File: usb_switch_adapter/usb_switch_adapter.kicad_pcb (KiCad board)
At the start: 2 copper layers, 19.4 x 33.3 mm, 12 parts, among them J1 USB-C Plug, J2 USB2.0-C_SMT, M2 Hole_M2_2.0, SW1 SW_Push, U1 CH217K, U2 CH32V003J4M6

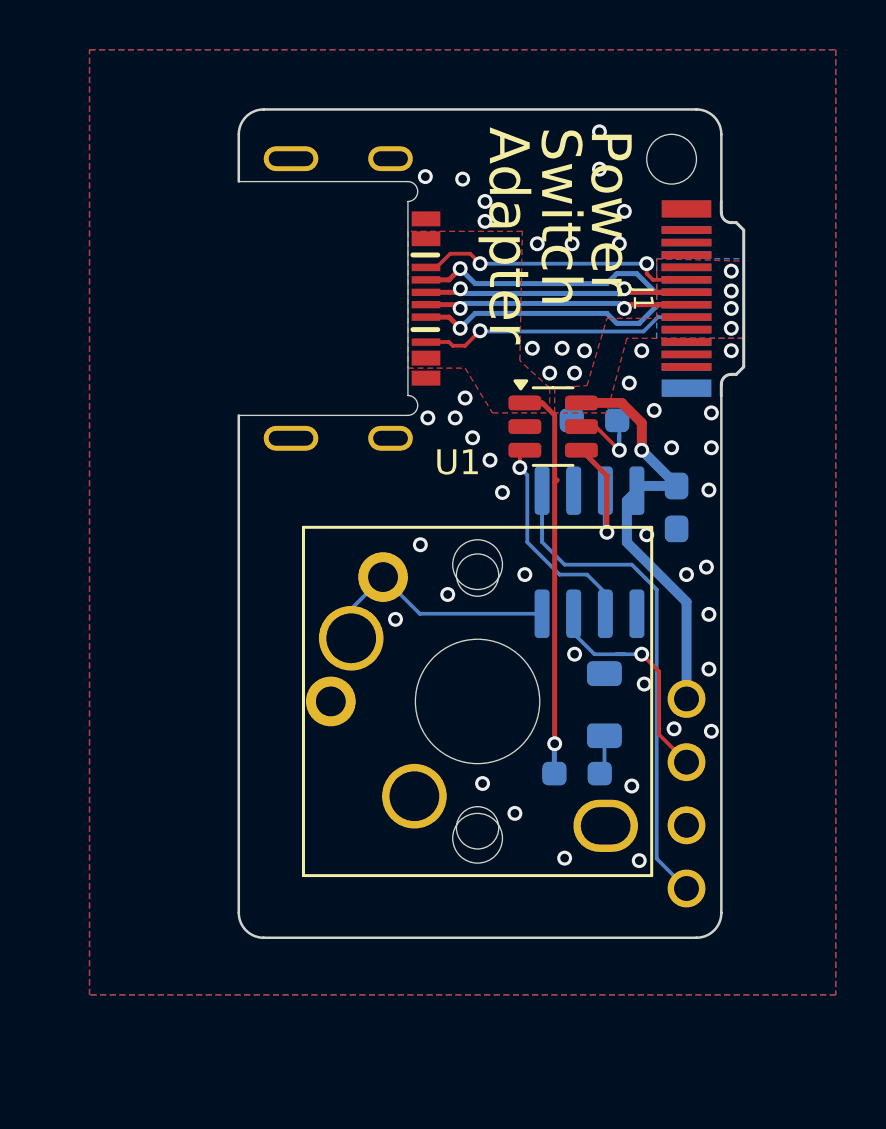
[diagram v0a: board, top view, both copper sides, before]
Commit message: usb-switch-adapter/1.0.0
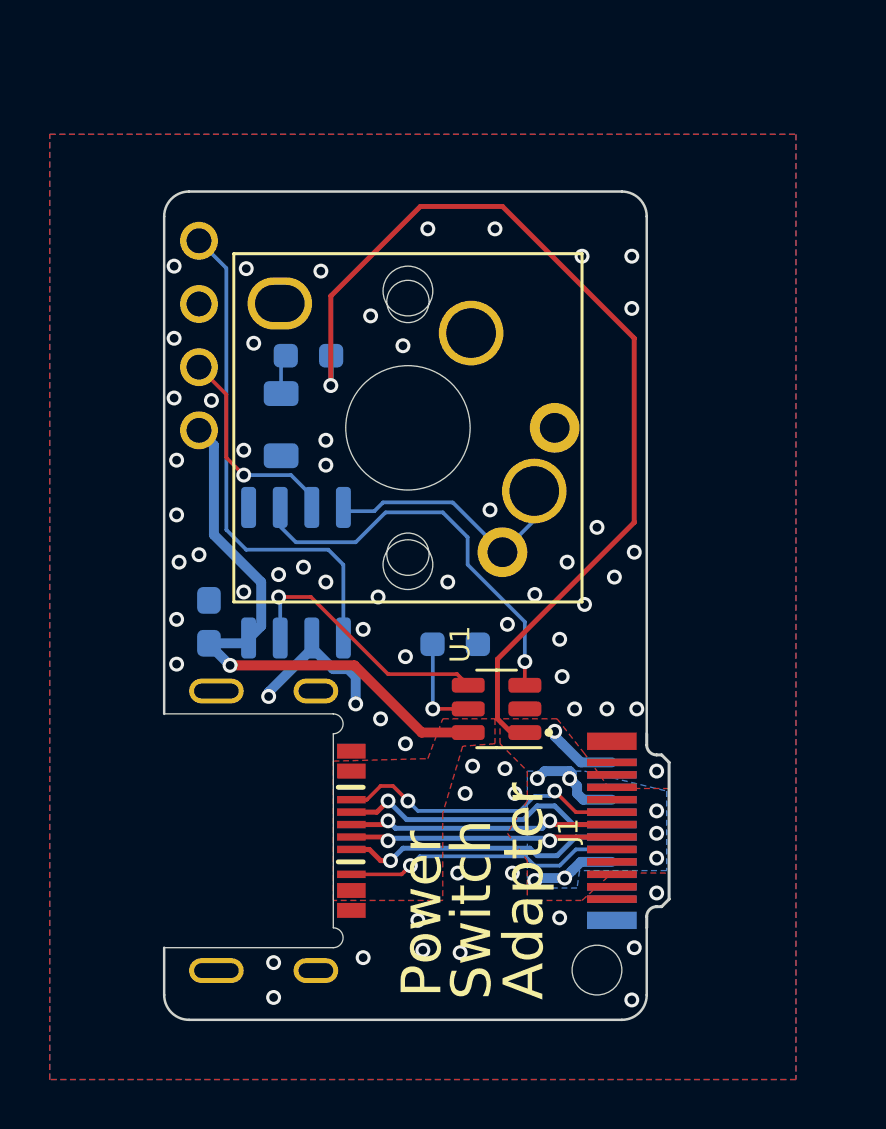
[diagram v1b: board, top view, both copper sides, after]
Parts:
- U1: footprint Package_TO_SOT_SMD:SOT-23-6 -> 74th:Package_SOT-23-6
- U2: footprint Package_SO:SOIC-8_3.9x4.9mm_P1.27mm -> 74th:Package_SOIC-8_3.9x4.9mm_P1.27mm
- moved M2 32.7 mm to (102.4, 64.0), turned to 180 degrees
- moved MISC-ICON 23.1 mm to (96.1, 59.6)
- moved CH1 22.4 mm to (86.4, 42.3), turned to 90 degrees
- moved J1 21.6 mm to (104.0, 58.4)
- moved J2 21.6 mm to (85.0, 58.4)
- moved R2 20.0 mm to (90.8, 39.3), turned to 180 degrees
- moved C1 19.4 mm to (86.8, 50.1), turned to 90 degrees
- moved D1 17.2 mm to (89.7, 42.1), turned to 90 degrees
- moved U2 11.8 mm to (90.3, 48.0), turned to 90 degrees
- moved U1 11.6 mm to (98.4, 53.5), turned to 180 degrees
- moved SW1 11.4 mm to (94.8, 42.2), turned to -90 degrees
- moved R1 10.6 mm to (96.7, 50.9), turned to 0 degrees
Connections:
- J1 pad A4: VBUS -> VCC
- J1 pad A9: VBUS -> VCC
- J1 pad B4: VBUS -> VCC
- J1 pad B9: VBUS -> VCC
- J2 pad A4/B9: VCC -> VBUS
- J2 pad A9/B4: VCC -> VBUS
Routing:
- net VCC: track 16.0 -> 46.6 mm, vias 1 -> 8
- net GND: track 0.00 -> 10.9 mm, vias 47 -> 66
- net /OUT_FLAG: track 8.73 -> 16.1 mm
- net VBUS: track 17.1 -> 23.2 mm, vias 5 -> 1
- net /OUT_EN: track 5.43 -> 10.6 mm
- net /SWDIO: track 9.26 -> 8.17 mm
- net /SWITCH: track 10.00 -> 9.18 mm
- added copper zone on B.Cu, net VCC
- removed copper zone on B.Cu, net VBUS
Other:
- outline, holes or cut-outs redrawn
- board text added: "74TH-G053-1.0.0"
- board text added: "G"
- board text added: "SD"
- board text added: "TX"
- board text added: "V"
- board text removed: "74TH-G53-1.0.0"
